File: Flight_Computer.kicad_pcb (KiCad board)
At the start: 4 copper layers, 100 x 66.2 mm, 67 parts, among them J1 PYRO, J2 PYRO, J3 Conn_01x04, J5 Conn_01x02_Pin, J6 Conn_01x09_Socket, J9 Conn_01x02_Pin, Q1 IRLZ44N, Q2 IRLZ44N, SW2 SW_Push, SW3 SW_Push, U1 TLV1117-33, U2 ESP32-S3-WROOM-1, U6 LPS22HH, U7 MAX-M8C, U8 LSM6DS3, U9 W25Q16JVSS

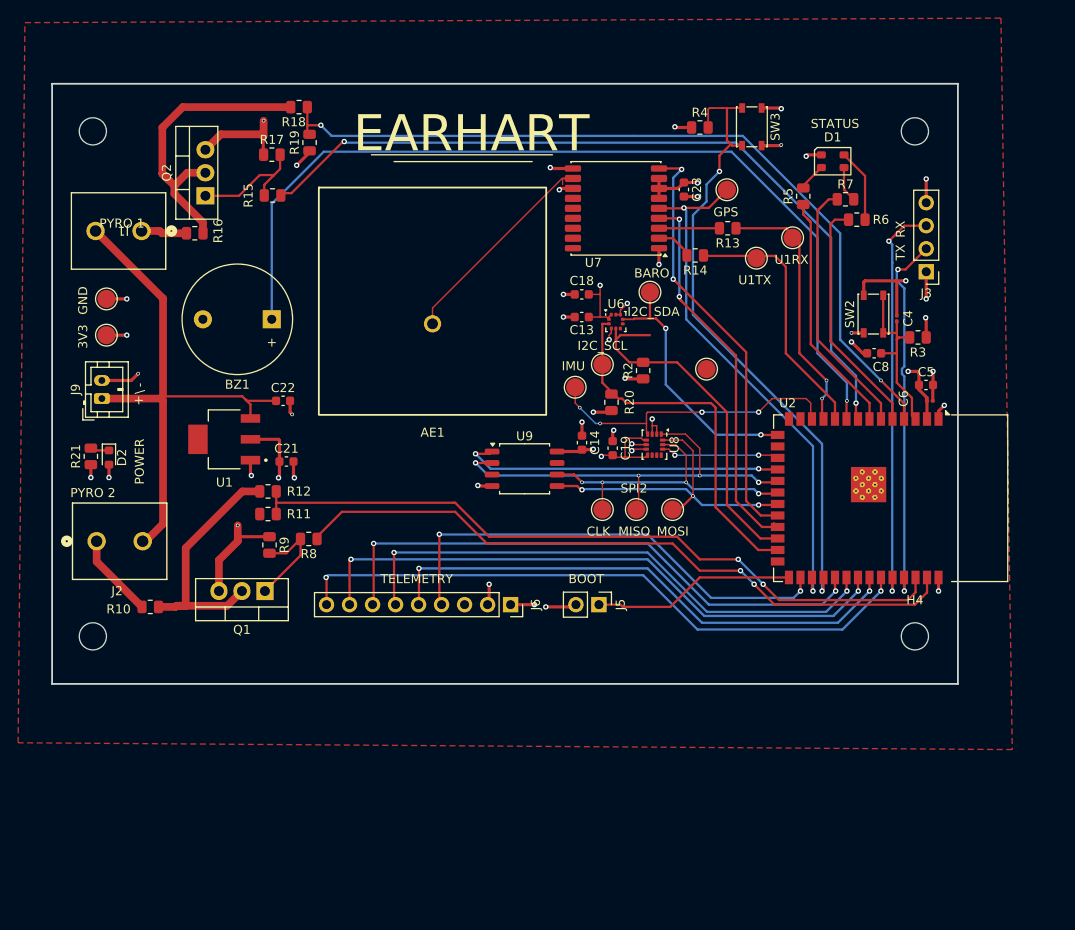
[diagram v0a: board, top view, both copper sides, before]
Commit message: Version 2 PCB
Updated layout, routing
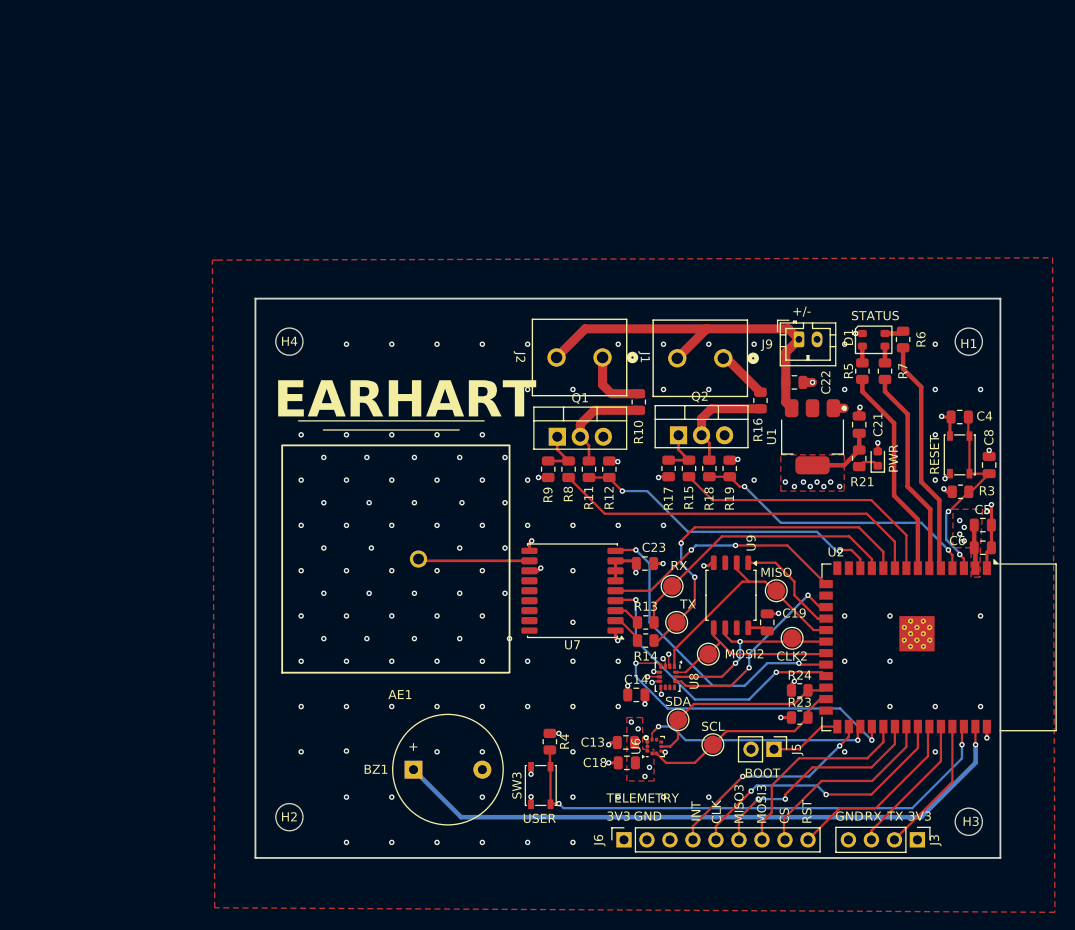
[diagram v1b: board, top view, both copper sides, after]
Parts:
- removed D2: LED, LED_SMD:LED_0603_1608Metric
- removed R2, R20: 4.7K, Resistor_SMD:R_0805_2012Metric
- removed SW2: SW_Push, Button_Switch_SMD:SW_SPST_PTS810
- removed TP1, TP10, TP11, TP12, TP13, TP15, TP16, TP2, TP4, TP6, TP7, TP9: TestPoint, TestPoint:TestPoint_Pad_D2.0mm
- added CLK2: TestPoint, TestPoint:TestPoint_Pad_D2.0mm, F.Cu at (199.2, 102.5)
- added MISO: TestPoint, TestPoint:TestPoint_Pad_D2.0mm, F.Cu at (197.5, 97.2)
- added MOSI2: TestPoint, TestPoint:TestPoint_Pad_D2.0mm, F.Cu at (190.0, 104.2)
- added PWR: LED, LED_SMD:LED_0603_1608Metric, F.Cu at (208.7, 82.6)
- added R23: 4.7K, Resistor_SMD:R_0805_2012Metric, F.Cu at (200.0, 111.2)
- added R24: 4.7K, Resistor_SMD:R_0805_2012Metric, F.Cu at (200.0, 108.2)
- added RESET: SW_Push, Button_Switch_SMD:SW_SPST_PTS810, F.Cu at (217.7, 82.2)
- added RX: TestPoint, TestPoint:TestPoint_Pad_D2.0mm, F.Cu at (186.0, 96.7)
- added SCL: TestPoint, TestPoint:TestPoint_Pad_D2.0mm, F.Cu at (190.5, 114.2)
- added SDA: TestPoint, TestPoint:TestPoint_Pad_D2.0mm, F.Cu at (186.6, 111.5)
- added TX: TestPoint, TestPoint:TestPoint_Pad_D2.0mm, F.Cu at (186.5, 100.7)
- C13, C14, C18, C19, C21, C22, C23, C5, C8: footprint Capacitor_SMD:C_0603_1608Metric -> Capacitor_SMD:C_0805_2012Metric
- C4, C6: footprint Capacitor_SMD:C_0201_0603Metric -> Capacitor_SMD:C_0805_2012Metric
- U1: footprint TLV1117-33CDCY:SOT230P700X180-4N -> Package_TO_SOT_SMD:SOT-223-3_TabPin2
- moved H1 99.4 mm to (218.7, 69.7)
- moved R21 84.8 mm to (206.6, 82.6), turned to -90 degrees
- moved J9 77.2 mm to (200.0, 69.5), turned to 0 degrees
- moved H3 76.4 mm to (218.7, 122.7)
- moved SW3 76.4 mm to (171.5, 118.7), turned to 90 degrees
- moved H4 76.3 mm to (143.7, 69.7)
- moved R4 69.8 mm to (172.5, 113.9), turned to -90 degrees
- moved J1 65.7 mm to (191.6, 71.6)
- moved R16 65.1 mm to (195.7, 76.2), turned to -90 degrees
- moved U1 65.0 mm to (201.5, 80.2), turned to -90 degrees
- moved C21 63.4 mm to (206.6, 78.9), turned to 90 degrees
- moved J3 62.7 mm to (213.0, 124.7), turned to -90 degrees
- moved R18 60.4 mm to (190.1, 83.7), turned to 90 degrees
- moved J2 59.4 mm to (178.3, 71.5), turned to 180 degrees
- moved R19 58.7 mm to (192.3, 83.7), turned to -90 degrees
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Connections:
- U2 pad 12: IMU_INT -> /SENSE_1
- U2 pad 15: BARO_INT -> GPS_EXTINT
- U2 pad 29: GPS_EXTINT -> BARO_INT
- U2 pad 30: /BUTT_0 -> IMU_INT
- U2 pad 38: /SENSE_1 -> /BUTT_0
- U2 pad 39: /PYRO_1 -> /BUZZER
- U2 pad 9: /BUZZER -> /PYRO_1
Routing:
- net /PYRO_2: track 88.8 -> 30.3 mm, vias 2 -> 0
- net /SENSE_2: track 90.3 -> 31.9 mm
- net GND: track 95.0 -> 40.3 mm, vias 34 -> 152
- net /TELE_RST: track 70.1 -> 20.4 mm, vias 2 -> 0
- net /TELE_CS: track 66.3 -> 21.4 mm, vias 2 -> 0
- net /SENSE_1: track 79.5 -> 34.8 mm
- net /MOSI3: track 63.0 -> 22.5 mm, vias 2 -> 0
- net /MISO3: track 61.3 -> 25.2 mm
- net +3.3V: track 61.6 -> 28.2 mm, vias 15 -> 25
- net /PYRO_1: track 74.9 -> 41.9 mm, vias 2 -> 0
- net GPS_EXTINT: track 58.1 -> 27.1 mm
- net /BUZZER: track 100.7 -> 70.7 mm
- net /MCU_RX: track 45.1 -> 15.2 mm, vias 2 -> 0
- net /SPI_CLK3: track 59.5 -> 30.6 mm
- net /TELE_INT: track 52.5 -> 23.9 mm
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- added copper zone on F.Cu, net +3.3V
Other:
- board size 100 x 66.2 mm -> 82.2 x 61.8 mm
- board text added: "+/-"
- board text added: "CS"
- board text added: "INT"
- board text added: "MISO3"
- board text added: "MOSI3"
- board text added: "R16"
- board text added: "RST"
- board text added: "USER"
- board text removed: "+"
- board text removed: "-"
- board text removed: "BARO"
- board text removed: "GPS"
- board text removed: "I2C_SCL"
- board text removed: "I2C_SDA"
- board text removed: "IMU"
- board text removed: "MISO"
- board text removed: "MOSI"
- board text removed: "POWER"
- board text removed: "PYRO 1"
- board text removed: "PYRO 2"
- board text removed: "SPI2"
- board text removed: "U1RX"
- board text removed: "U1TX"
- board text removed: "\"
